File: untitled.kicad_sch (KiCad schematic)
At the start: 59 parts, among them J1 Conn_01x04_Pin, J10 Conn_01x03_Pin, J2 USB_B_Micro, J3 Conn_01x02_Pin, J4 Conn_01x02_Pin, J6 Screw_Terminal_01x02, J9 Screw_Terminal_01x02, U1 STM32F767ZITx, U2 MAX17501AATB+, U5 AT24C256, U8 AMS1117-3.3, Y1 16MHz

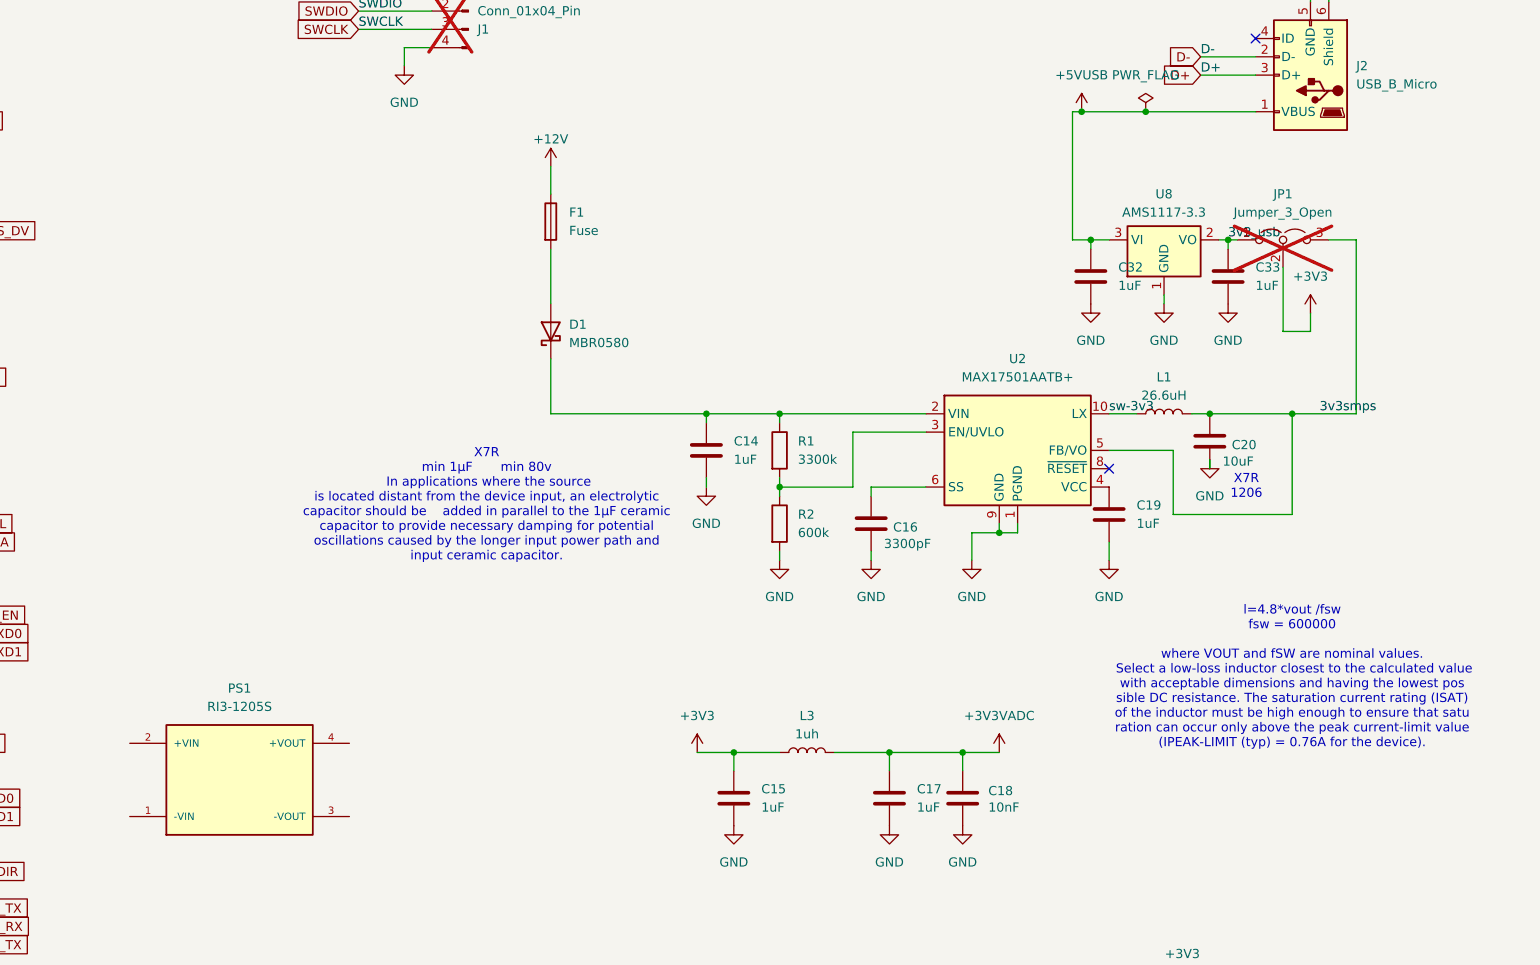
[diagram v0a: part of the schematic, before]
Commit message: Autosave
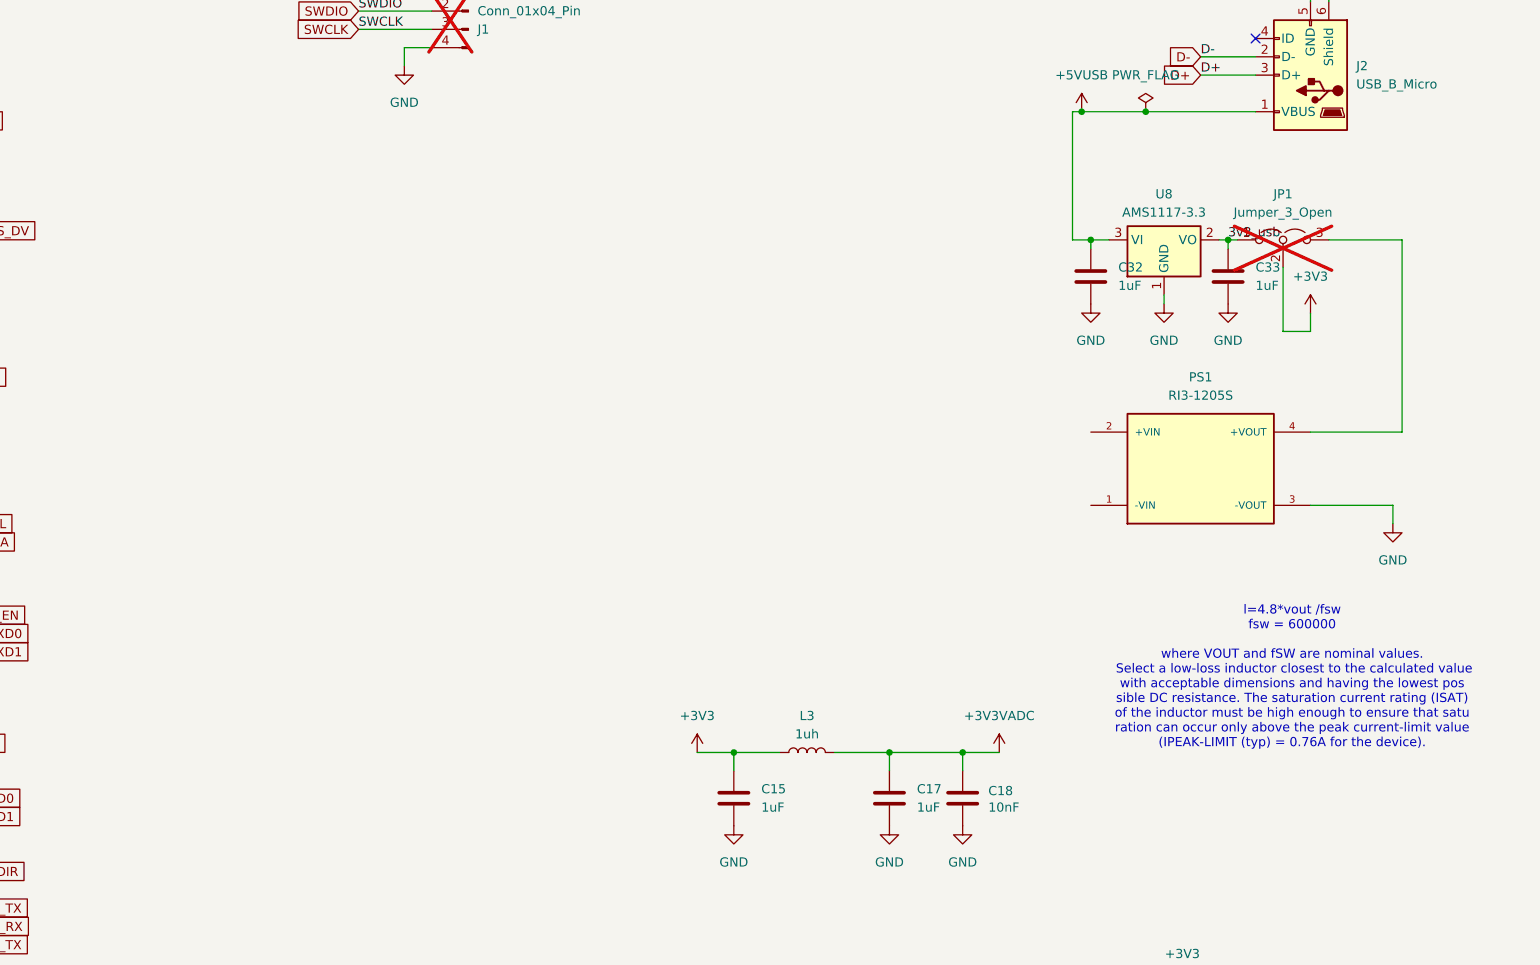
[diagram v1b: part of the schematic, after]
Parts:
- removed C14: 1uF, Capacitor_SMD:C_1206_3216Metric, symbol Device:C
- removed C16: 3300pF, Capacitor_SMD:C_0402_1005Metric, symbol Device:C
- removed C19: 1uF, Capacitor_SMD:C_0603_1608Metric, symbol Device:C
- removed C20: 10uF, Capacitor_SMD:C_0603_1608Metric, symbol Device:C
- removed D1: MBR0580, Diode_SMD:D_SOD-123, symbol Diode:MBR0580
- removed F1: Fuse, Fuse:Fuse_1206_3216Metric, symbol Device:Fuse
- removed L1: 26.6uH, Inductor_SMD:L_Changjiang_FNR4018S, symbol Device:L
- removed R1: 3300k, Resistor_SMD:R_0402_1005Metric, symbol Device:R
- removed R2: 600k, Resistor_SMD:R_0402_1005Metric, symbol Device:R
- removed U2: MAX17501AATB+, Package_DFN_QFN:TDFN-10-1EP_2x3mm_P0.5mm_EP0.9x2mm, symbol Regulator_Switching:MAX17501AxTB
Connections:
- net 3v3smps is gone; now on an unnamed net: JP1.3 (B)
- net GND: now also PS1.3 (-VOUT)
- no-connect marks 92 -> 91
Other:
- note removed: "X7R 1206"
- note removed: "X7R min 1μF min 80v In applications where the source is located distant from the device input, an electrolytic capacitor should be added in parallel to the 1μF ceramic capacitor to provide necessary damping for potential oscillations caused by the longer input power path and input ceramic capacitor."
- moved on the sheet: PS1
